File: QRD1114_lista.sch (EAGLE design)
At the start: 18 parts

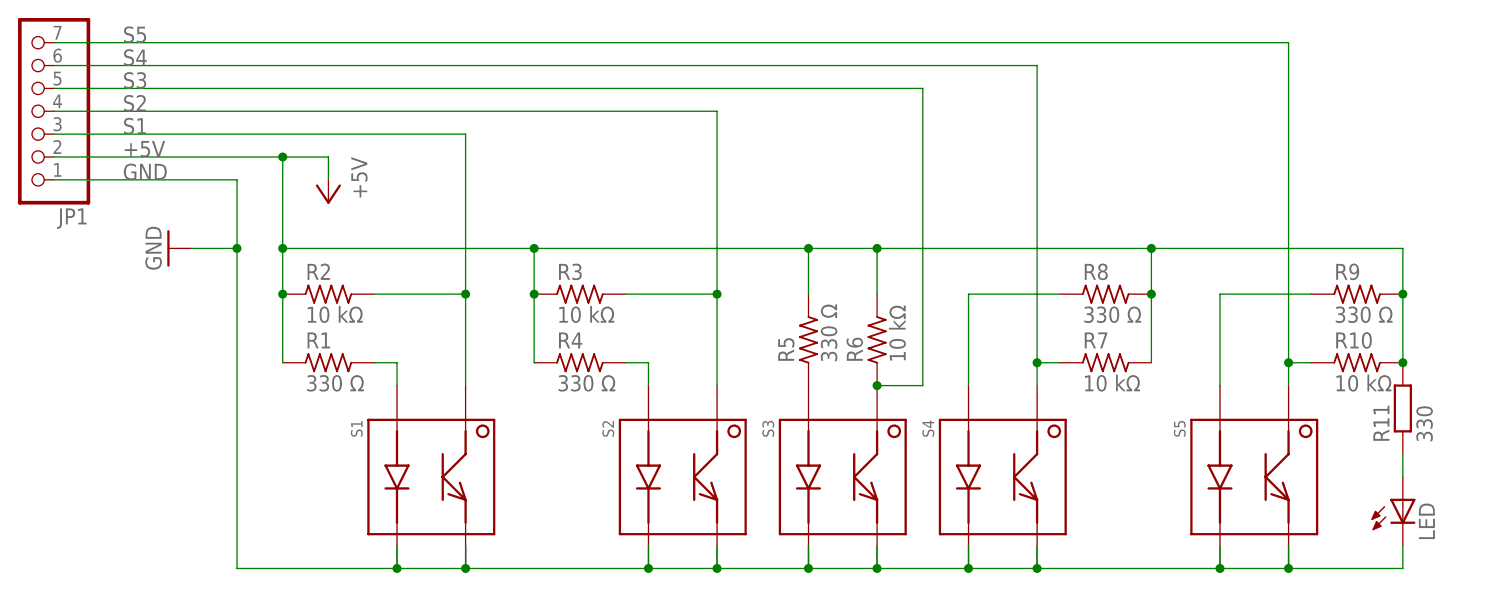
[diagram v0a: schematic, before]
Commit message: Add files via upload
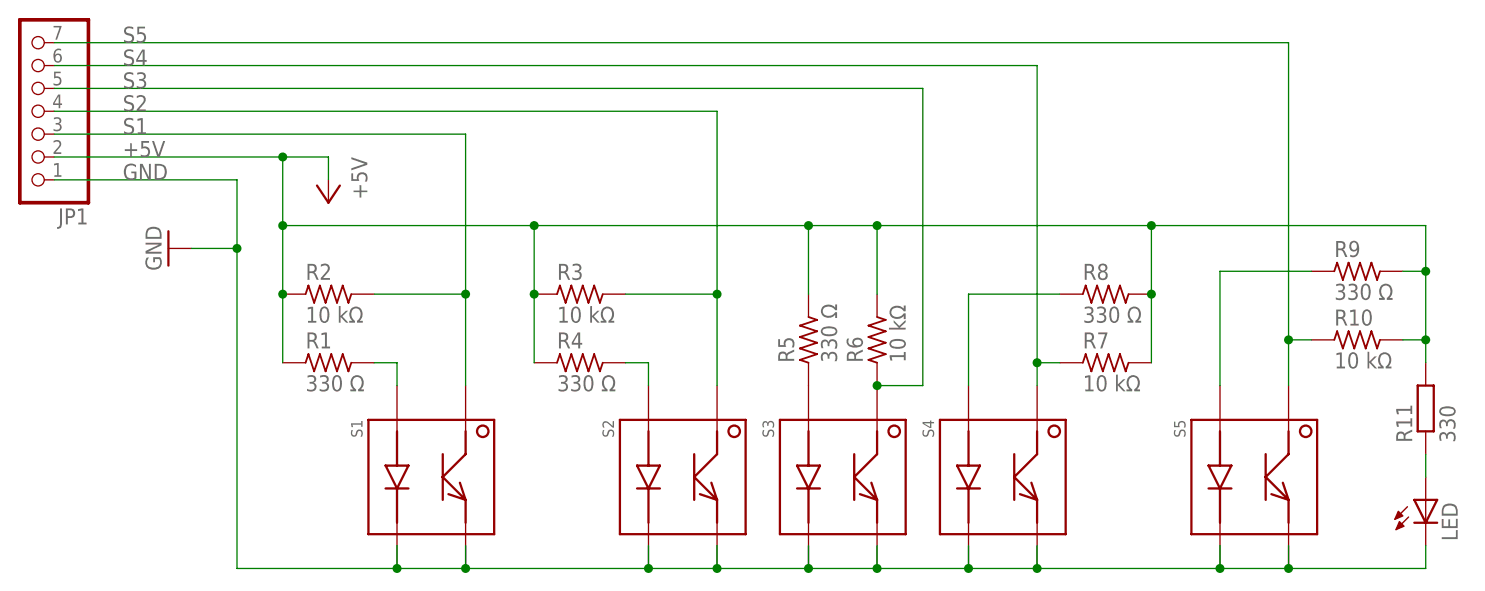
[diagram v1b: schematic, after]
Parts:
- LED: device led:LEDCHIPLED-0603-TTW -> led:LEDSML0603
- R11: device resistor:R-EU_R0805 -> resistor:R-EU_R0603
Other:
- moved on the sheet: LED, R10, R11, R9
